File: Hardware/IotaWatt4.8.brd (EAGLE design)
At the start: 87 x 67.9 mm, 53 parts

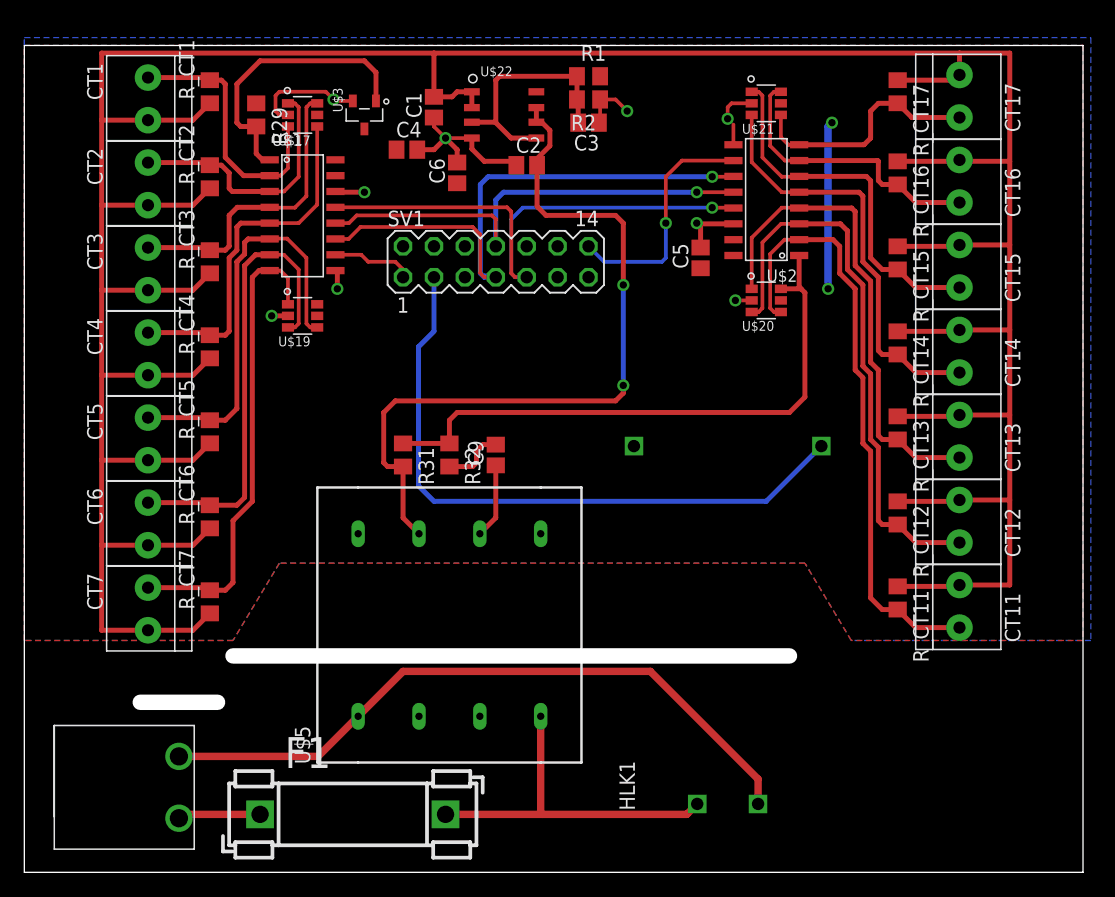
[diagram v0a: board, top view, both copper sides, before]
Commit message: fixed some minor errors on the board
fixed some minor errors on the board
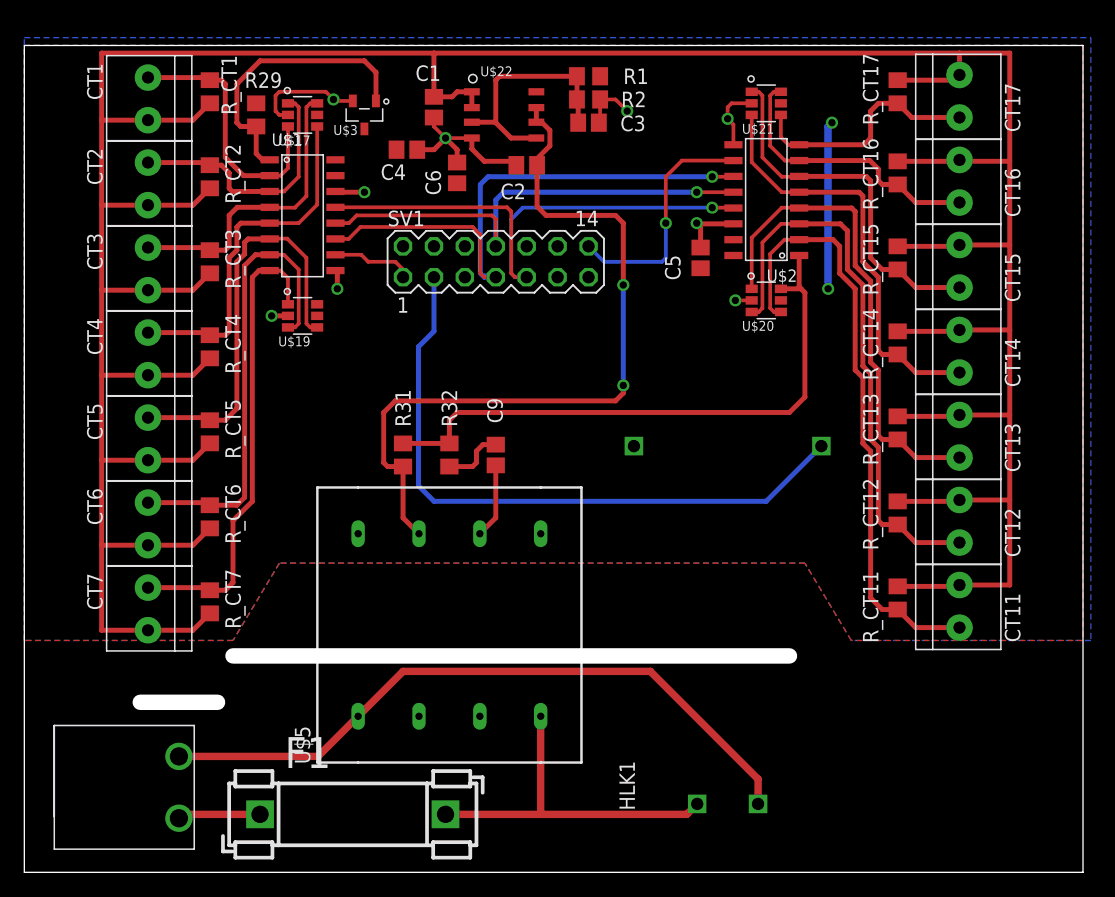
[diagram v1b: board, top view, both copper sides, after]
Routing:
- net GND: track 44.3 -> 45.0 mm
